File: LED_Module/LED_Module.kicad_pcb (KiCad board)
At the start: 2 copper layers, 53.5 x 30 mm, 9 parts, among them P3 CONN_02X04, P4 CONN_02X04, U1 AL8805WS

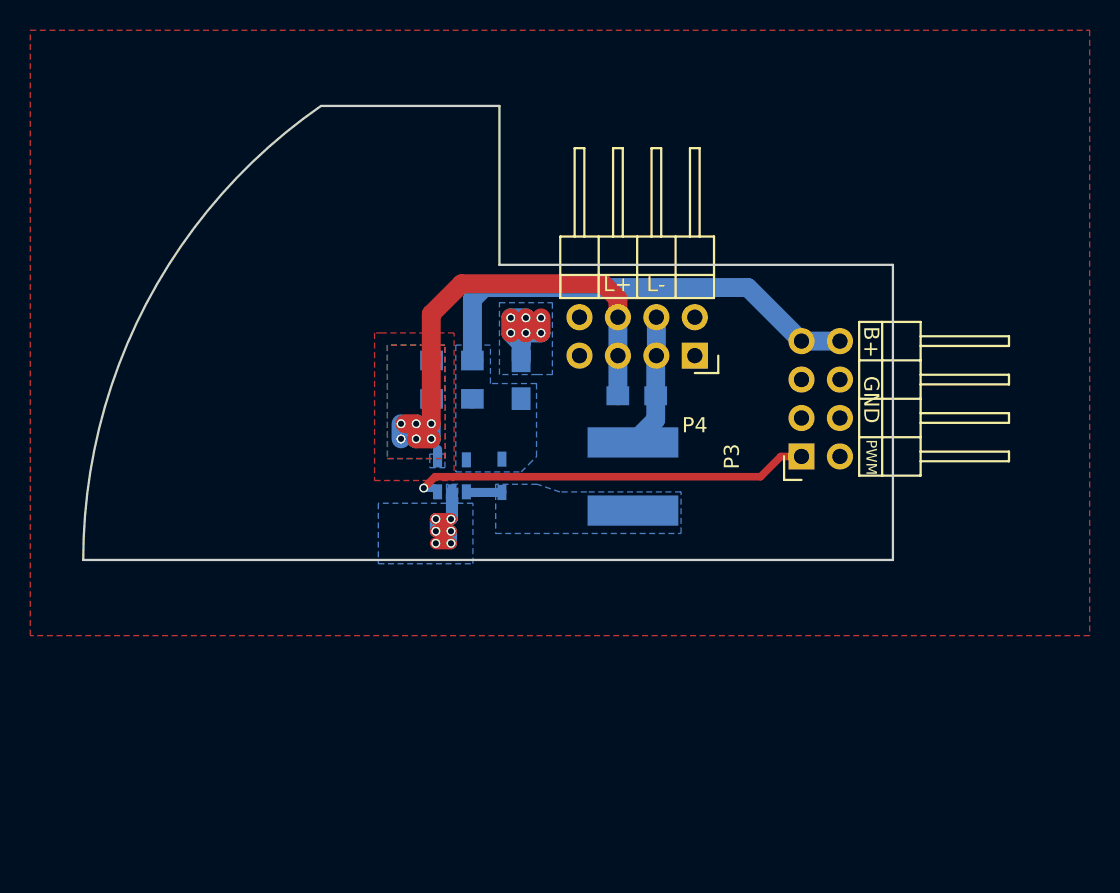
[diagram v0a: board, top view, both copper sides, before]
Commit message: LED Modulization
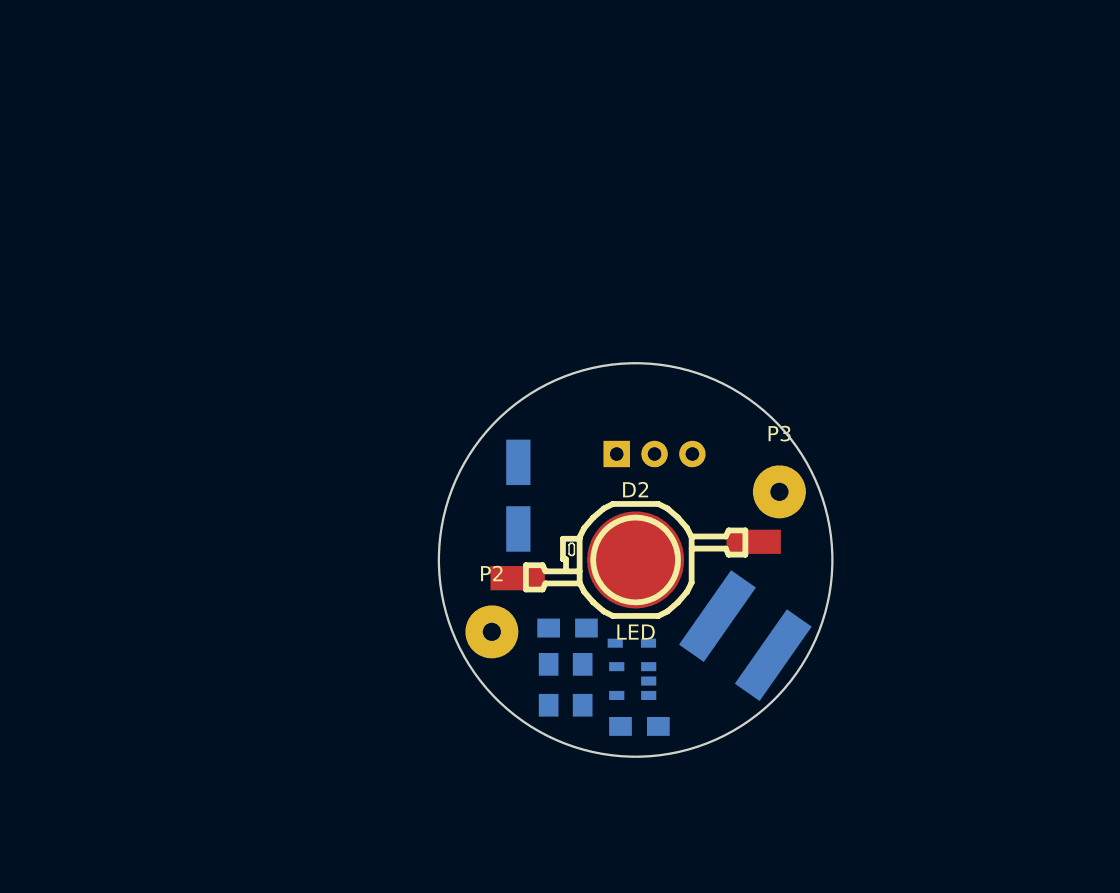
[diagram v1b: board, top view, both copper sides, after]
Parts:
- removed P4: CONN_02X04, KiCad_Footprint:Socket_Strip_Angled_2x04
- added C2: C, Capacitors_SMD:c_elec_5x4.5, B.Cu at (92.2, 95.8)
- added D2: LED, KiCad_Footprint:Power_LED, F.Cu at (100.0, 100.0)
- added P1: CONN_01X03, Connectors_JST:JST_XH_B03B-XH-A_03x2.50mm_Straight, B.Cu at (98.8, 93.0)
- added P2: CONN_01X01, Wire_Pads:SolderWirePad_single_1-2mmDrill, F.Cu at (90.5, 104.8)
- P3: value CONN_02X04 -> CONN_01X01; footprint KiCad_Footprint:Socket_Strip_Angled_2x04 -> Wire_Pads:SolderWirePad_single_1-2mmDrill
- moved R3 22.4 mm to (94.2, 108.2), turned to 270 degrees
- moved C1 21.8 mm to (100.2, 111.0)
- moved R1 20.8 mm to (96.5, 108.2), turned to 270 degrees
- moved U1 18.1 mm to (99.8, 108.0), turned to 270 degrees
- moved C3 16.7 mm to (95.5, 104.5), turned to 0 degrees
- moved D1 14.0 mm to (99.8, 105.5), turned to 0 degrees
- moved L1 12.9 mm to (107.2, 105.0), turned to 325 degrees
- moved P3 2.76 mm to (109.5, 95.5), turned to 0 degrees
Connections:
- P3 pad 1: /CTRL_PWM -> /LED1-
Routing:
- net /LED1+: track 32.7 -> 0.00 mm, vias 6 -> 0
- net /V_BAT: track 30.2 -> 0.00 mm
- net /CTRL_PWM: track 26.8 -> 0.00 mm, vias 1 -> 0
- net GND: track 13.6 -> 0.00 mm, vias 12 -> 0
- net /LED1-: track 8.92 -> 0.00 mm
- net Net-(D1-Pad2): track 2.37 -> 0.00 mm
- removed copper zone on B.Cu, net /LED1+
- removed copper zone on F.Cu, net /LED1+
- removed copper zone on B.Cu, net /V_BAT
- removed copper zone on B.Cu, net GND
- removed copper zone on F.Cu, net GND
- removed copper zone on B.Cu, net Net-(D1-Pad2)
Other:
- board size 53.5 x 30 mm -> 26 x 26 mm
- board text removed: "B+"
- board text removed: "GND"
- board text removed: "L+"
- board text removed: "L-"
- board text removed: "PWM"

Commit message: PCB square shape
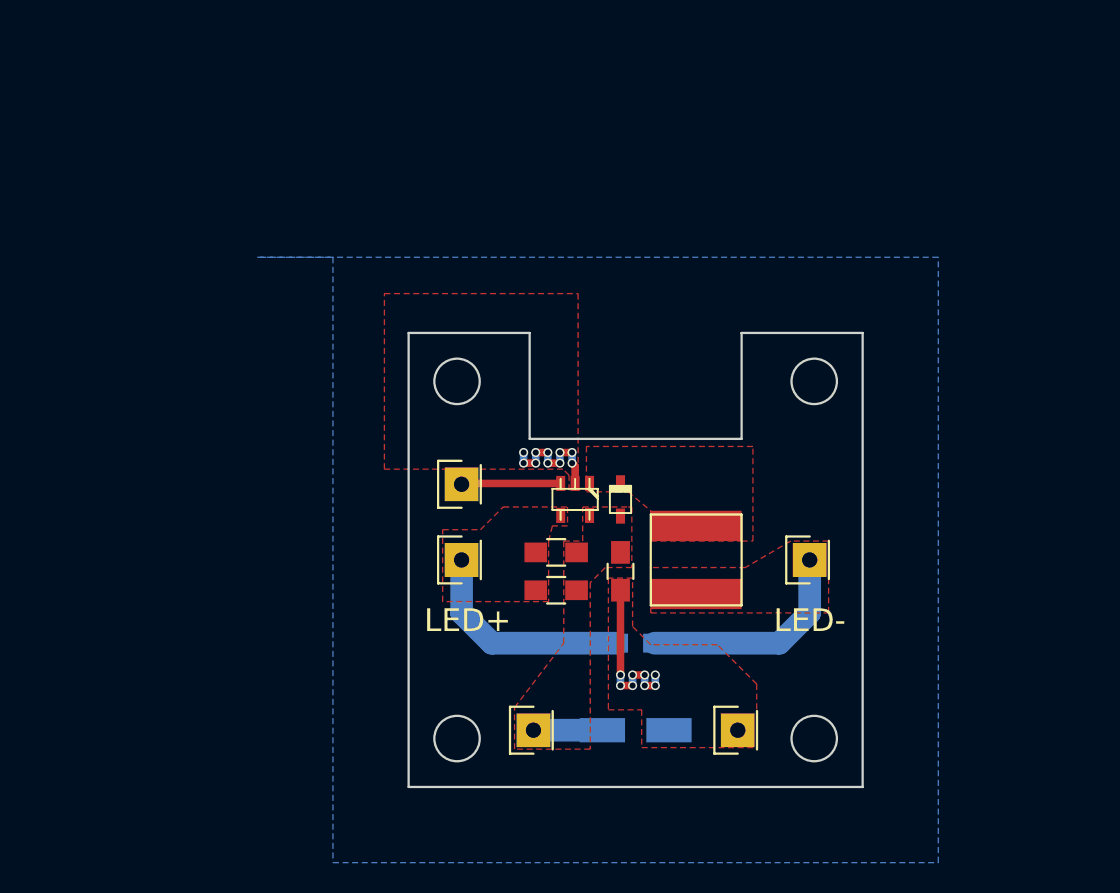
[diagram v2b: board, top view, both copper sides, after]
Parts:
- removed D2: LED, KiCad_Footprint:Power_LED
- added P4: CONN_01X01, Socket_Strips:Socket_Strip_Straight_1x01, F.Cu at (88.5, 100.0)
- added P5: CONN_01X01, Socket_Strips:Socket_Strip_Straight_1x01, F.Cu at (111.5, 100.0)
- C3, D1, L1, R1, R3, U1: moved to F.Cu
- P1: value CONN_01X03 -> CONN_01X01; footprint Connectors_JST:JST_XH_B03B-XH-A_03x2.50mm_Straight -> Socket_Strips:Socket_Strip_Straight_1x01; moved to F.Cu
- P2, P3: footprint Wire_Pads:SolderWirePad_single_1-2mmDrill -> Socket_Strips:Socket_Strip_Straight_1x01
- moved P3 21.0 mm to (88.5, 95.0)
- moved P1 19.9 mm to (106.8, 111.2)
- moved C2 17.3 mm to (100.0, 111.2), turned to 0 degrees
- moved U1 12.6 mm to (96.0, 96.0), turned to 180 degrees
- moved D1 9.53 mm to (99.0, 96.0), turned to 90 degrees
- moved R1 8.92 mm to (94.8, 99.5), turned to 180 degrees
- moved P2 7.06 mm to (93.2, 111.2)
- moved R3 6.27 mm to (94.8, 102.0), turned to 180 degrees
- moved L1 5.96 mm to (104.0, 100.0), turned to 270 degrees
- moved C1 5.51 mm to (100.0, 105.5)
- moved C3 5.13 mm to (99.0, 100.8), turned to 90 degrees
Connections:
- P2 pad 1: /LED1+ -> /V_BAT
- P3 pad 1: /LED1- -> /CTRL_PWM
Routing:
- net GND: track 0.00 -> 18.8 mm, vias 0 -> 18
- net /LED1-: track 0.00 -> 14.6 mm
- net /LED1+: track 0.00 -> 14.6 mm
- net /CTRL_PWM: track 0.00 -> 6.57 mm
- net /V_BAT: track 0.00 -> 4.55 mm
- added copper zone on F.Cu, net /LED1+
- added copper zone on F.Cu, net /LED1-
- added copper zone on F.Cu, net /V_BAT
- added copper zone on B.Cu, net GND
- added copper zone on F.Cu, net GND
- added copper zone on F.Cu, net Net-(D1-Pad2)
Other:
- board size 26 x 26 mm -> 30 x 30 mm
- net class Default: trace_width 0.6 -> 0.5
- board text added: "GND"
- board text added: "LED+"
- board text added: "LED-"
- board text added: "PWM"
- board text added: "V+"
